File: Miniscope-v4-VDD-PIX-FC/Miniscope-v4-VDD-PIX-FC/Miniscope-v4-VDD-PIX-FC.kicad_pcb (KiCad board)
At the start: 2 copper layers, 7.2 x 6.5 mm, 7 parts, among them J1 Conn_01x01, J2 Conn_01x01, J3 Conn_01x01, U1 MCP1711

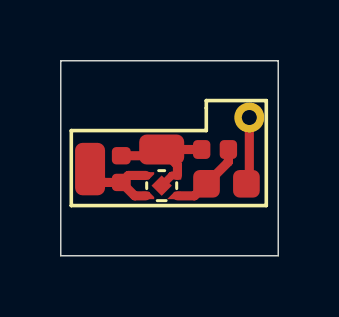
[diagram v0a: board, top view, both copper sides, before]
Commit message: Finalize v0.1 VDD-PIX FC for fab at OSHPark and PCBWay
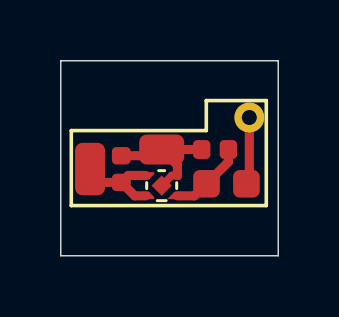
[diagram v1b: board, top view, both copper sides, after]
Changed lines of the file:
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@@
   (general
     (thickness 0.381)
-    (drawings 17)
+    (drawings 20)
     (tracks 19)
     (zones 0)
@@
     (visible_elements FFFFFF7F)
     (pcbplotparams
-      (layerselection 0x010fc_ffffffff)
+      (layerselection 0x018fc_ffffffff)
       (usegerberextensions false)
       (usegerberattributes true)
@@
 ) (width 0))
       ))
+    (model ${KICAD_AHARONI_LAB}/Modules/Package_QFN.pretty/MCP1711.step
+      (at (xyz 0 0 0))
+      (scale (xyz 1 1 1))
+      (rotate (xyz -90 0 0))
+    )
   )
   (module .Connector:Conn_1x1_700_Circular_Pad (layer F.Cu)
@@
     )
   )
+  (gr_line (start 144 97) (end 144 101) (layer Eco2.User) (width 0.15))
+  (gr_line (start 151.25 97) (end 144 97) (layer Eco2.User) (width 0.15))
+  (gr_line (start 151.25 101) (end 151.25 97) (layer Eco2.User) (width 0.15))
+  (gr_line (start 144 101) (end 151.25 101) (layer Eco2.User) (width 0.15))
   (gr_line (start 150.25 97) (end 150.25 98) (layer B.SilkS) (width 0.12))
   (gr_text V_PIX (at 149 98.75) (layer B.SilkS)
@@
     (effects (font (size 1 1) (thickness 0.15)))
   )
-  (gr_line (start 148.8516 95.8276) (end 148.8516 96.0776) (layer F.SilkS) (width 0.12))
+  (gr_line (start 148.8516 95.8276) (end 148.8516 96.8276) (layer F.SilkS) (width 0.12))
   (gr_line (start 150.8516 95.8276) (end 148.8516 95.8276) (layer F.SilkS) (width 0.12))
   (gr_line (start 150.8516 99.3276) (end 150.8516 95.8276) (layer F.SilkS) (width 0.12))
   (gr_line (start 144.3516 96.8276) (end 144.3516 99.3276) (layer F.SilkS) (width 0.12))
-  (gr_line (start 148.8516 96.0776) (end 148.8516 96.8276) (layer F.SilkS) (width 0.12))
   (gr_line (start 148.8516 96.8276) (end 144.3516 96.8276) (layer F.SilkS) (width 0.12))
   (gr_line (start 150.8516 99.3276) (end 144.3516 99.3276) (layer F.SilkS) (width 0.12))
